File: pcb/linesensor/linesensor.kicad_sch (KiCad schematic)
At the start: 3 parts, among them J1 Conn_01x03_Socket

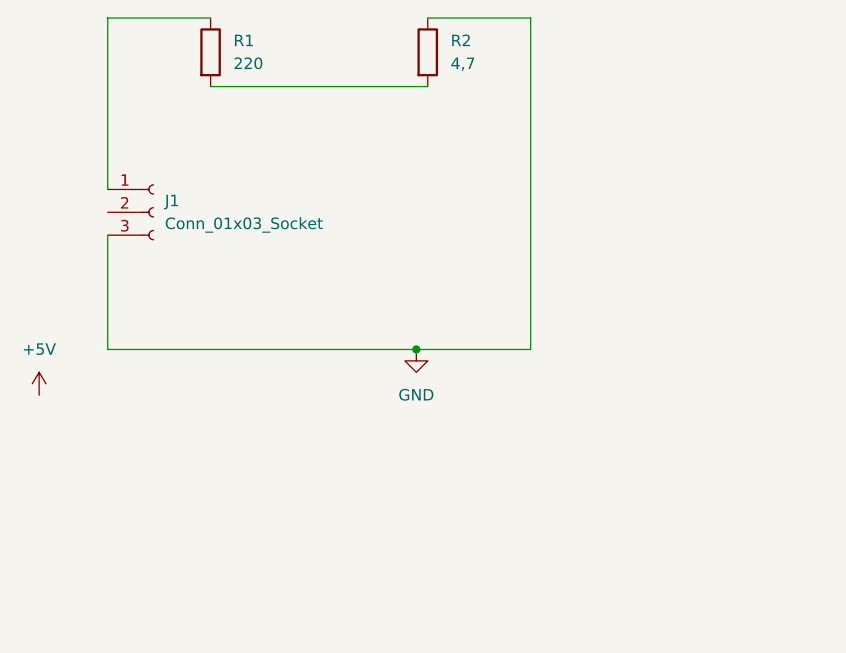
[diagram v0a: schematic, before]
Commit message: linesensor new
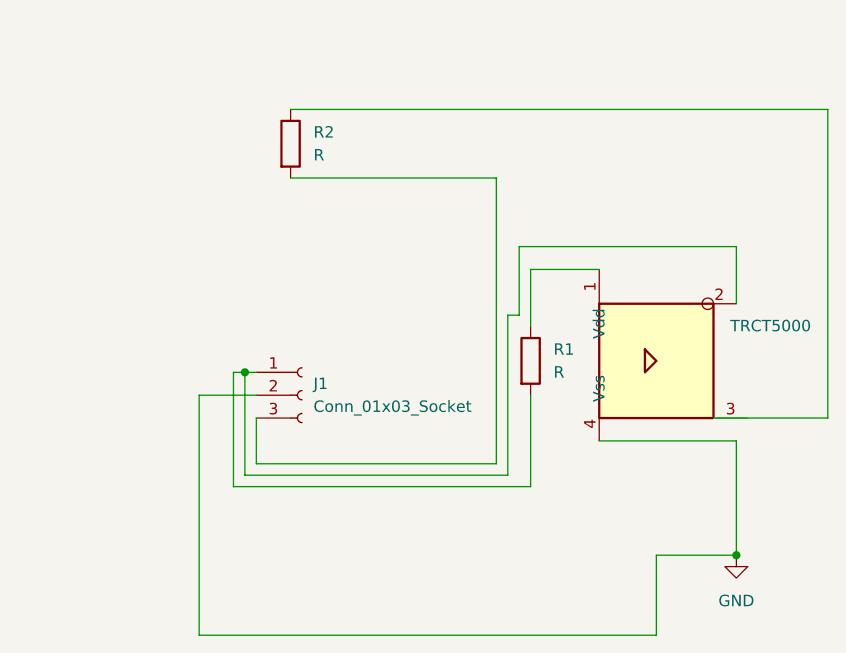
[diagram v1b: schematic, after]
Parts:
- added U1: TRCT5000, Library:CRT5000, symbol 4xxx_IEEE:4049
- R1: value 220 -> R; footprint Resistor_THT:R_Axial_DIN0207_L6.3mm_D2.5mm_P7.62mm_Horizontal -> Resistor_THT:R_Axial_DIN0309_L9.0mm_D3.2mm_P12.70mm_Horizontal
- R2: value 4,7 -> R; footprint Resistor_THT:R_Axial_DIN0207_L6.3mm_D2.5mm_P7.62mm_Horizontal -> Resistor_THT:R_Axial_DIN0309_L9.0mm_D3.2mm_P12.70mm_Horizontal
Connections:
- net GND: now also J1.2 (Pin_2), U1.4 (Vss); no longer J1.3 (Pin_3), R2.1
- net at J1.1 (Pin_1): now also R1.2, U1.2; no longer R1.1
- net at R2.2: now also J1.3 (Pin_3); no longer R1.2
- new net: R2.1, U1.3
- new net: R1.1, U1.1 (Vdd)
